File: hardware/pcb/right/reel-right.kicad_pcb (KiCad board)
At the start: 2 copper layers, 145 x 88.1 mm, 47 parts, among them J1 Conn_01x02, J3 Conn_01x05, SW1 SW_Push, SW10 SW_Push, SW11 SW_Push, SW12 SW_Push, SW13 SW_Push, SW14 SW_Push, SW15 SW_Push, SW16 SW_Push, SW17 SW_Push, SW18 SW_Push, SW19 SW_Push, SW2 SW_Push, SW22 SW_SPDT, SW3 SW_Push, SW4 SW_Push, SW5 SW_Push, SW6 SW_Push, SW7 SW_Push, SW8 SW_Push, SW9 SW_Push

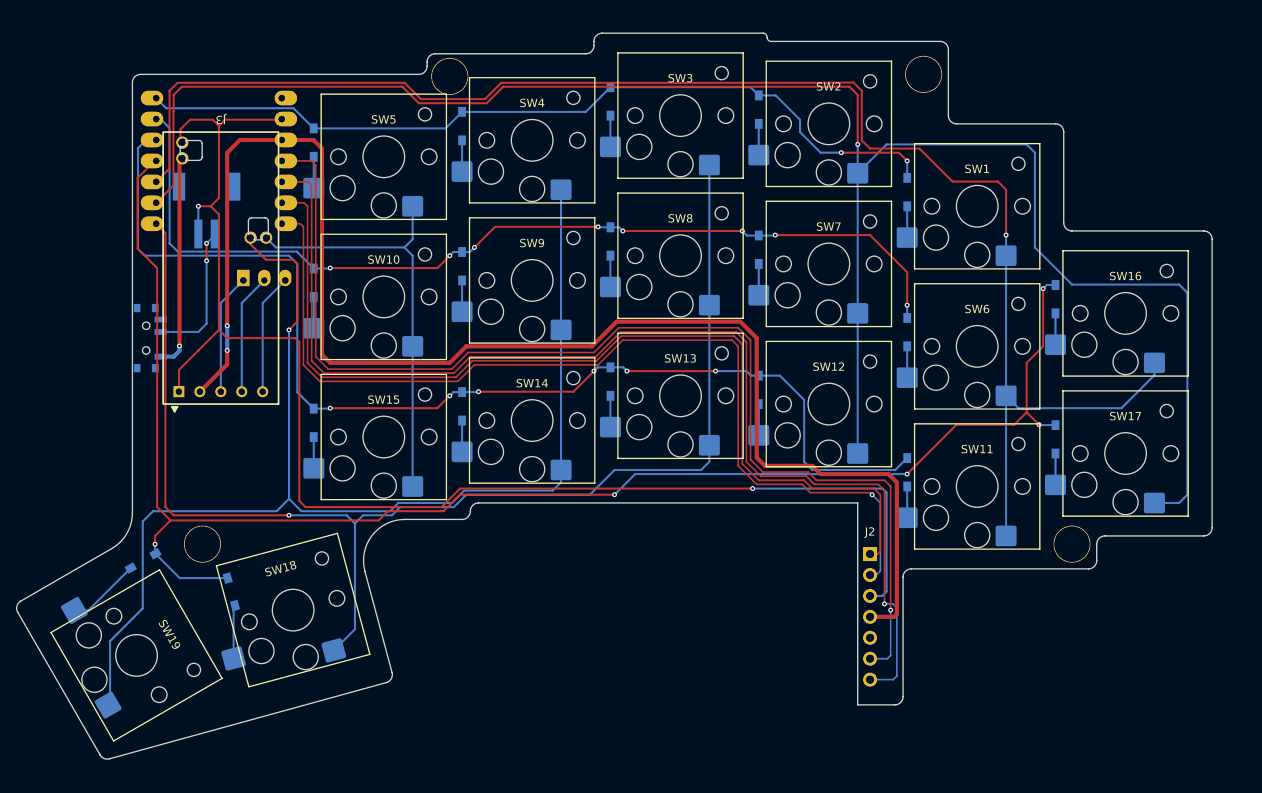
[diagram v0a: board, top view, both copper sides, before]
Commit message: Update PCB and side switch research
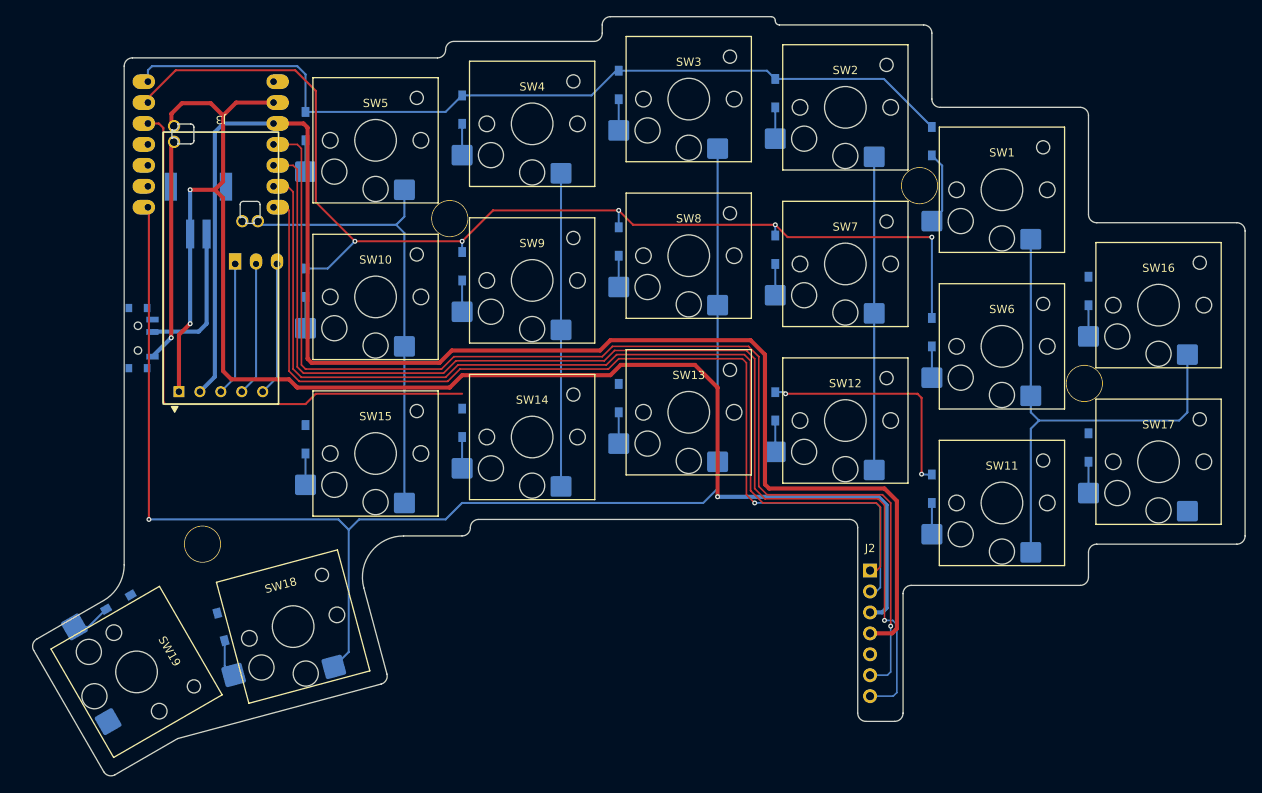
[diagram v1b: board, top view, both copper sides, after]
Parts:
- moved Ref** 19.6 mm to (165.0, 88.0)
- moved Ref** 17.2 mm to (88.0, 68.0)
- moved Ref** 13.5 mm to (145.0, 64.0)
- moved D1 6.87 mm to (146.5, 55.8)
- moved D19 5.83 mm to (50.2, 113.1)
- moved D18 4.43 mm to (59.5, 114.8)
- moved D16 4.12 mm to (165.5, 74.0)
- moved D17 4.12 mm to (165.5, 93.0)
- moved SW16 4.12 mm to (174.0, 78.5)
- moved SW17 4.12 mm to (174.0, 97.5)
- moved D11 3.61 mm to (146.5, 98.0)
- moved SW1 3.61 mm to (155.0, 64.5)
- moved SW11 3.61 mm to (155.0, 102.5)
- moved D6 3.00 mm to (146.5, 79.0)
- moved SW6 3.00 mm to (155.0, 83.5)
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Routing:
- net Row3: track 192.2 -> 0.00 mm, vias 5 -> 0
- net Col1: track 227.5 -> 38.0 mm, vias 1 -> 0
- net Col0: track 187.9 -> 64.2 mm, vias 1 -> 0
- net Col3: track 149.2 -> 38.0 mm, vias 1 -> 0
- net Row2: track 137.5 -> 100.8 mm, vias 6 -> 2
- net Row1: track 116.8 -> 138.3 mm, vias 8 -> 5
- net GND: track 171.3 -> 188.2 mm, vias 2 -> 3
- net Col2: track 157.2 -> 168.2 mm
- net 3.3V: track 176.1 -> 181.4 mm, vias 2 -> 0
- net Row0: track 101.4 -> 106.6 mm, vias 2 -> 0
- net Net-(D1-A): track 3.80 -> 9.01 mm
- net Net-(D19-A): track 8.98 -> 4.73 mm
- net nCS: track 118.8 -> 123.0 mm
- net Col4: track 51.8 -> 55.5 mm
- net SDIO: track 139.7 -> 142.9 mm
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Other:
- board size 145 x 88.1 mm -> 147.1 x 92.1 mm
